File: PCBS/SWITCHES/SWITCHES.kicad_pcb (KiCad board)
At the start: 2 copper layers, 30 x 15 mm, 22 parts, among them J1 Conn_01x03_Pin, J2 Conn_01x02_Socket, J3 Conn_01x02_Socket, J6 Conn_01x02_Socket, J7 Conn_01x02_Socket, J8 Conn_01x03_Socket, U1 CD4043BPWR

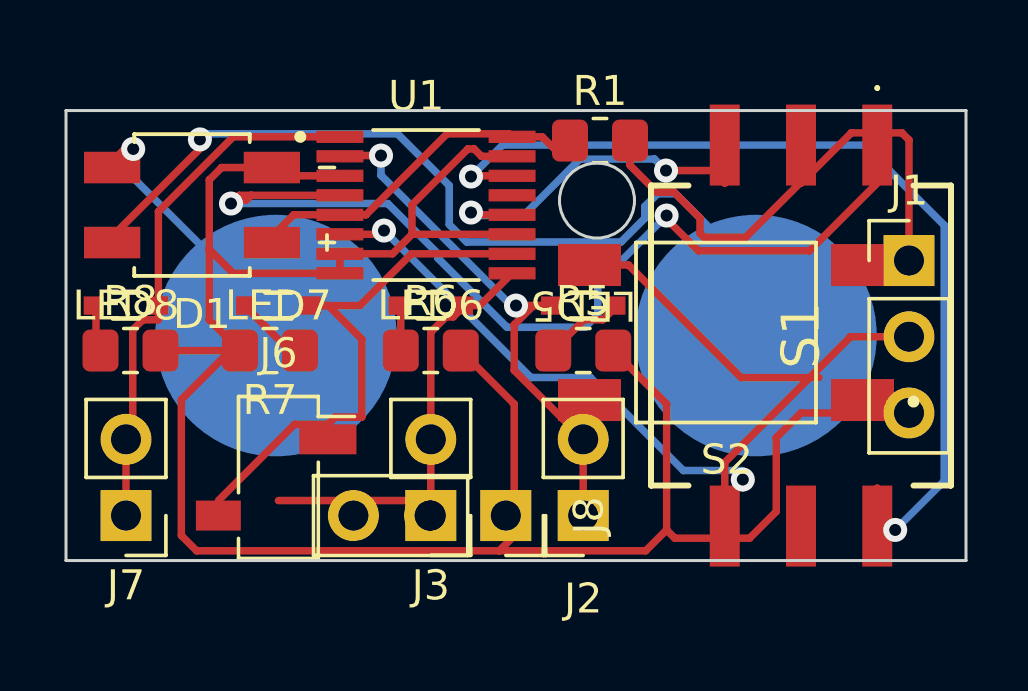
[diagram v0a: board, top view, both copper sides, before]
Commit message: Rev1 board/mux/switches/output
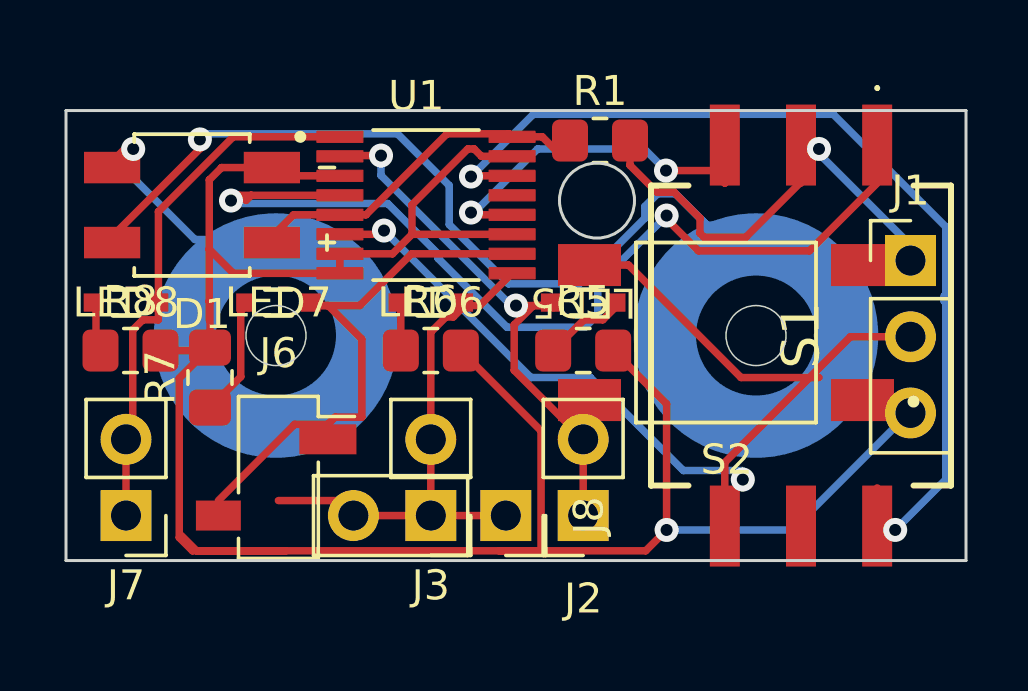
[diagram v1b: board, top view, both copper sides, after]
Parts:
- added G***: LOGO, DigitalLogicFootprints:HBBLogo, B.Cu at (165.1, 93.5)
- moved R7 2.19 mm to (144.8, 88.9), turned to 90 degrees
- moved LED5 0.10 mm to (157.2, 86.4)
- moved LED6 0.10 mm to (152.2, 86.4)
- moved LED7 0.10 mm to (147.1, 86.4)
- moved LED8 0.10 mm to (142.0, 86.4)
- moved J1 0.05 mm to (168.2, 85.0)
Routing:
- net Net-(J5-PWR): track 32.0 -> 36.8 mm
- net GND: track 79.6 -> 83.8 mm, vias 0 -> 1
- net /OUTPUT1: track 14.2 -> 16.8 mm
- net Net-(J4-PWR): track 9.56 -> 12.1 mm
- net Net-(LED7-Pad1): track 2.56 -> 4.06 mm
- net /VCC_RES: track 18.0 -> 16.7 mm, vias 0 -> 1
- net /DEBOUNCE3: track 31.2 -> 32.1 mm
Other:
- board text added: "Jonathan Hess (jetsama.com)"
- board text added: "SWITCHES PCB REV 1"
